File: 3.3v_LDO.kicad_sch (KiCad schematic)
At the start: 9 parts

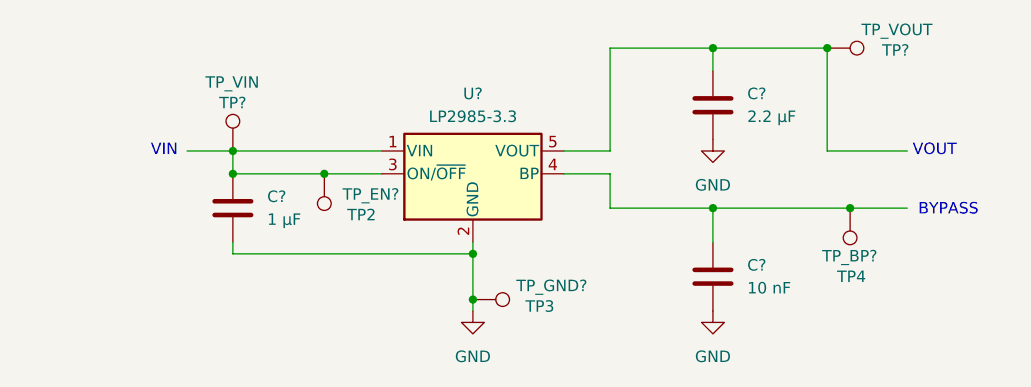
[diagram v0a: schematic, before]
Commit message: Add LDO schematic + layout
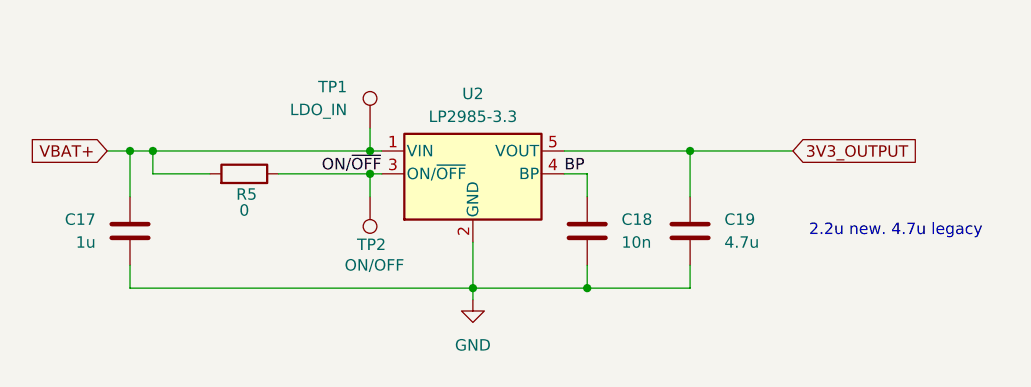
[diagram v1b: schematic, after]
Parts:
- removed C?: 10 nF, symbol Device:C
- removed C?: 2.2 µF, symbol Device:C
- removed C?: 1 µF, symbol Device:C
- removed TP?: TP_VIN, symbol Connector:TestPoint
- removed TP?: TP_VOUT, symbol Connector:TestPoint
- removed TP_BP?: TP4, symbol Connector:TestPoint
- removed TP_EN?: TP2, symbol Connector:TestPoint
- removed TP_GND?: TP3, symbol Connector:TestPoint
- added C17: 1u, Capacitor_SMD:C_0603_1608Metric, symbol Device:C
- added C18: 10n, Capacitor_SMD:C_0402_1005Metric, symbol Device:C
- added C19: 4.7u, Capacitor_SMD:C_0603_1608Metric, symbol Device:C
- added R5: 0, Resistor_SMD:R_0603_1608Metric, symbol Device:R
- added TP1: LDO_IN, TestPoint:TestPoint_THTPad_D1.0mm_Drill0.5mm, symbol Connector:TestPoint
- added TP2: ON/OFF, TestPoint:TestPoint_THTPad_D1.0mm_Drill0.5mm, symbol Connector:TestPoint
- gave numbers to parts that had none: 1
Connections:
- net GND: now also C17.2, C18.2, C19.2
- net ON/~{OFF}: now reaches U2.3 (ON/~{OFF})
- net ON/~{OFF}: now also R5.1, TP2.1; no longer U2.1 (VIN)
- net BP: now reaches U2.4 (BP)
- net BP: now also C18.1
- net 3V3_OUTPUT: now reaches U2.5 (VOUT)
- net 3V3_OUTPUT: now also C19.1
- new net VBAT+: C17.1, R5.2, TP1.1, U2.1 (VIN)
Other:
- note added: "2.2u new. 4.7u legacy"
- note removed: "BYPASS"
- note removed: "VIN"
- note removed: "VOUT"
